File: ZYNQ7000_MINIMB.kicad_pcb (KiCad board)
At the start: 4 copper layers, 86 x 68.9 mm, 125 parts, among them J1 Conn_02x50_Odd_Even, J10 Conn_02x20_Odd_Even, J11 USB_A_Stacked, J12 Conn_01x40, J2 Conn_02x50_Odd_Even, J3 ZYNQ_JTAG, J5 USB_C_Receptacle_USB2.0, J6 HDMI_A, J8 USB_A_Stacked, J9 USB_C_Receptacle_USB2.0, SW2 SW_DIP_x01, SW5 SW_DIP_x02, U1 HR911130A, U2 CP2102N-A01-GQFN28, U4 TXS02612RTWR, U5 TF_Card, U6 TXS0108EPWR, U7 USB3320, U8 TPS2051BDBV, U9 GL850G, Y1 24Mhz, Y2 12Mhz

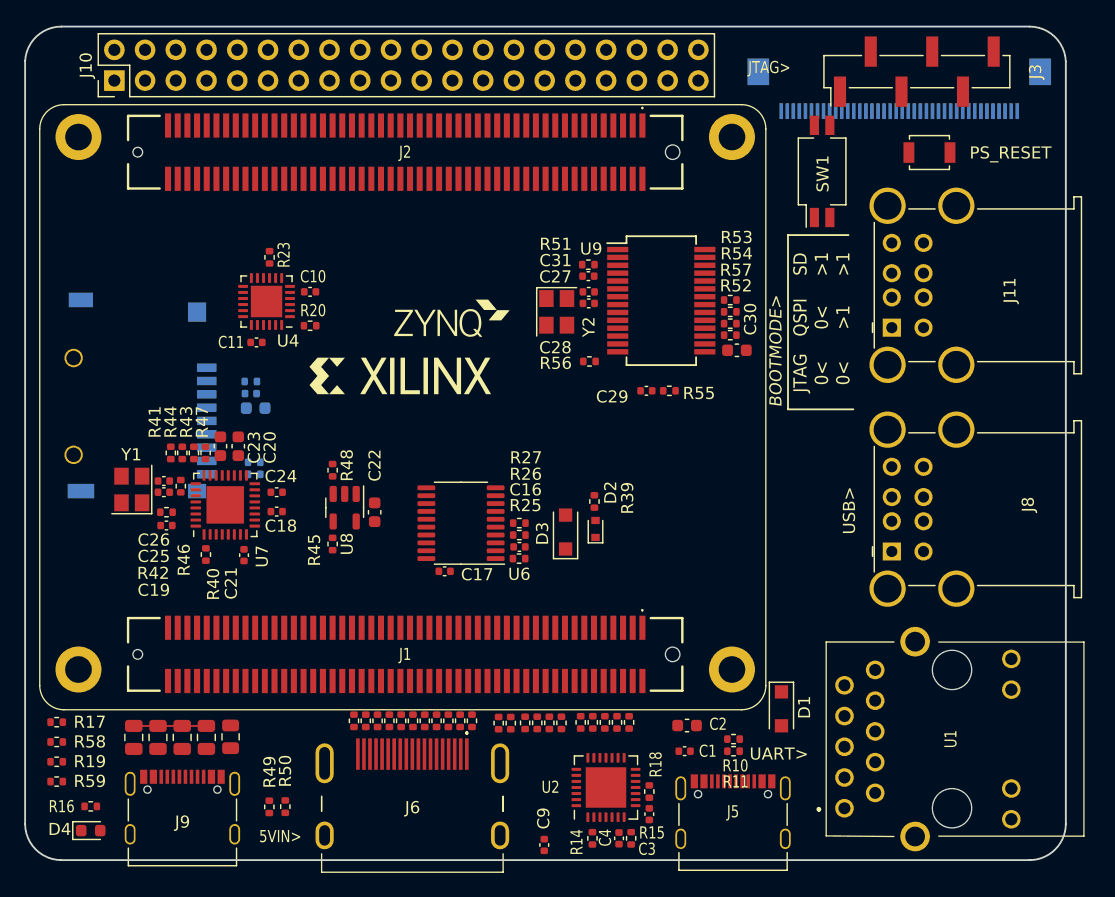
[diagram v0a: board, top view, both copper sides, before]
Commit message: update layout
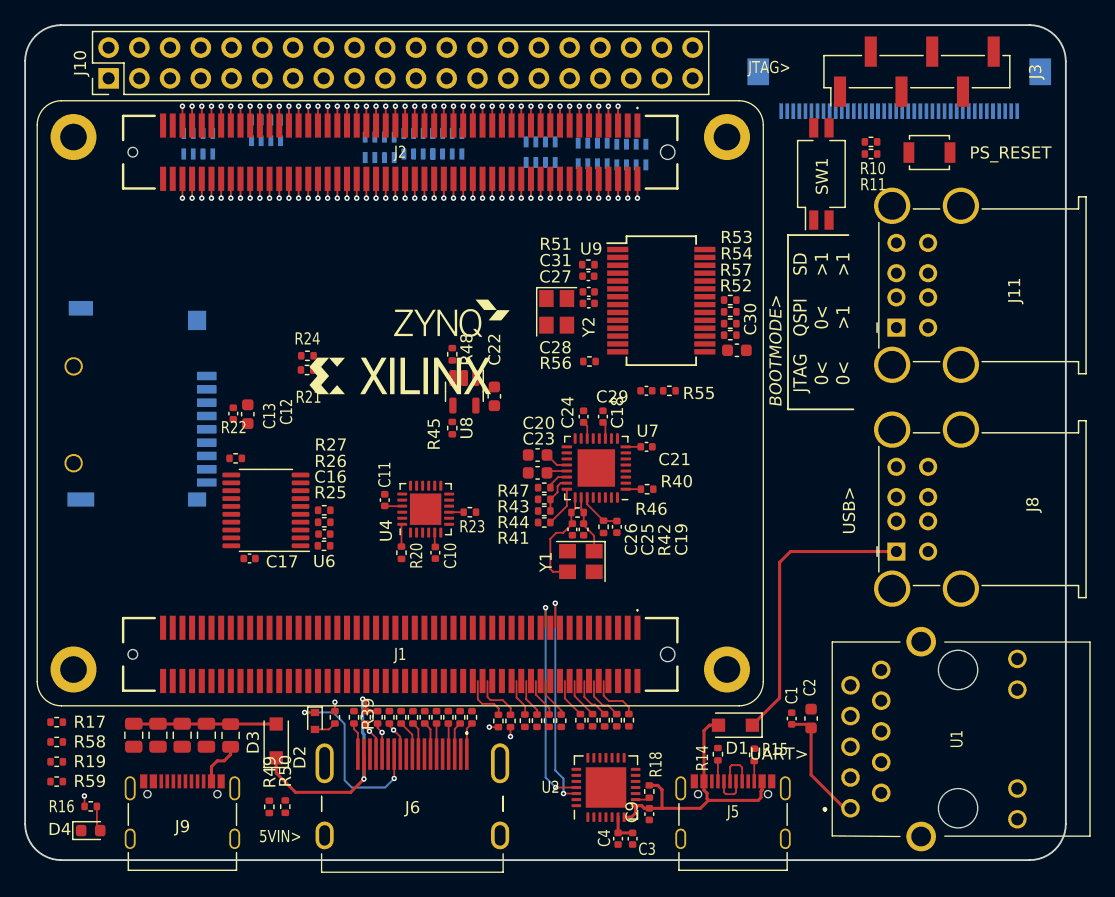
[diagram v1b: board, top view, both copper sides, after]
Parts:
- added RN1: R_Pack04, Resistor_SMD:R_Array_Concave_4x0603, B.Cu at (120.1, 61.7)
- added RN2: R_Pack04, Resistor_SMD:R_Array_Concave_4x0603, B.Cu at (116.9, 61.6)
- added RN3: R_Pack04, Resistor_SMD:R_Array_Concave_4x0603, B.Cu at (104.9, 60.8)
- added RN4: R_Pack04, Resistor_SMD:R_Array_Concave_4x0603, B.Cu at (112.6, 61.5)
- added RN5: R_Pack04, Resistor_SMD:R_Array_Concave_4x0603, B.Cu at (102.5, 60.8)
- added RN6: R_Pack04, Resistor_SMD:R_Array_Concave_4x0603, B.Cu at (99.3, 61.1)
- added RN7: R_Pack04, Resistor_SMD:R_Array_Concave_4x0603, B.Cu at (84.3, 60.8)
- added RN8: R_Pack04, Resistor_SMD:R_Array_Concave_4x0603, B.Cu at (89.9, 59.7)
- C12, C13, R21, R22, R24: moved to F.Cu
- moved R10 50.6 mm to (139.9, 60.6)
- moved R11 50.6 mm to (139.9, 61.6)
- moved Y1 37.6 mm to (115.9, 95.3), turned to 180 degrees
- moved C19 37.2 mm to (118.9, 92.5), turned to -90 degrees
- moved R40 36.9 mm to (121.4, 89.3), turned to 180 degrees
- moved R42 36.1 mm to (117.8, 92.5), turned to -90 degrees
- moved C25 34.8 mm to (116.2, 92.7), turned to -90 degrees
- moved C21 34.4 mm to (121.3, 85.8), turned to 0 degrees
- moved C26 34.0 mm to (115.2, 92.7), turned to -90 degrees
- moved R46 32.9 mm to (115.7, 91.3), turned to 0 degrees
- moved R41 31.4 mm to (112.9, 92.1), turned to 0 degrees
- moved U7 30.8 mm to (117.2, 87.6), turned to 180 degrees
- moved R44 30.3 mm to (112.9, 91.2), turned to 180 degrees
- moved D3 29.5 mm to (90.8, 110.2)
- moved R43 29.2 mm to (112.9, 90.2), turned to 180 degrees
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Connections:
- C3 pad 2: GND2 -> GND
- C4 pad 2: GND2 -> GND
- C9 pad 2: GND2 -> GND
- J10 pad 10: /B35_L7N -> Net-(J10-Pad10)
- J10 pad 13: /B34_L7P -> Net-(J10-Pad13)
- J10 pad 14: /B34_L7N -> Net-(J10-Pad14)
- J10 pad 15: /B34_L10P -> Net-(J10-Pad15)
- J10 pad 16: /B34_L10N -> Net-(J10-Pad16)
- J10 pad 17: /B34_L8P -> Net-(J10-Pad17)
- J10 pad 18: /B34_L8N -> Net-(J10-Pad18)
- J10 pad 19: /B34_L9P -> Net-(J10-Pad19)
- J10 pad 20: /B34_L9N -> Net-(J10-Pad20)
- J10 pad 21: /B34_L2P -> Net-(J10-Pad21)
- J10 pad 22: /B34_L2N -> Net-(J10-Pad22)
- J10 pad 23: /B34_L1P -> Net-(J10-Pad23)
- J10 pad 24: /B34_L1N -> Net-(J10-Pad24)
- J10 pad 27: /B13_L11P -> Net-(J10-Pad27)
- J10 pad 28: /B13_L11N -> Net-(J10-Pad28)
- J10 pad 29: /B13_L19P -> Net-(J10-Pad29)
- J10 pad 3: /B35_L11P -> Net-(J10-Pad3)
- J10 pad 30: /B13_L19N -> Net-(J10-Pad30)
- J10 pad 31: /B13_L18P -> Net-(J10-Pad31)
- J10 pad 32: /B13_L18N -> Net-(J10-Pad32)
- J10 pad 33: /B13_L16P -> Net-(J10-Pad33)
- J10 pad 34: /B13_L16N -> Net-(J10-Pad34)
- J10 pad 35: /B13_L14P -> Net-(J10-Pad35)
- J10 pad 36: /B13_L14N -> Net-(J10-Pad36)
- J10 pad 37: /B13_L13P -> Net-(J10-Pad37)
- J10 pad 38: /B13_L13N -> Net-(J10-Pad38)
- J10 pad 4: /B35_L11N -> Net-(J10-Pad4)
- J10 pad 5: /B35_L21P -> Net-(J10-Pad5)
- J10 pad 6: /B35_L21N -> Net-(J10-Pad6)
- J10 pad 7: /B35_L9P -> Net-(J10-Pad7)
- J10 pad 8: /B35_L9N -> Net-(J10-Pad8)
- J10 pad 9: /B35_L7P -> Net-(J10-Pad9)
- J5 pad A1: GND2 -> GND
- J5 pad A12: GND2 -> GND
- J5 pad B1: GND2 -> GND
- J5 pad B12: GND2 -> GND
- J5 pad S1: GND2 -> GND
- R14 pad 1: GND2 -> GND
- R15 pad 1: GND2 -> GND
- U2 pad 29: GND2 -> GND
- U2 pad 3: GND2 -> GND
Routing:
- net /USB_5V: track 0.00 -> 24.0 mm
- net Net-(C3-Pad1): track 0.00 -> 23.9 mm
- net /hdmi/HDMI5VD: track 0.00 -> 20.4 mm, vias 0 -> 2
- net /B0MIO14: track 0.00 -> 19.1 mm, vias 0 -> 2
- net /B0MIO15: track 0.00 -> 18.6 mm, vias 0 -> 2
- net /B35_L3P: track 0.00 -> 15.9 mm, vias 0 -> 2
- net Net-(C1-Pad1): track 0.00 -> 9.50 mm
- net Net-(C26-Pad1): track 0.00 -> 8.68 mm
- net GND: track 0.00 -> 8.00 mm, vias 0 -> 5
- net /VDD5VD: track 6.00 -> 12.6 mm, vias 0 -> 1
- net /VDD1V8D: track 0.00 -> 5.31 mm
- net Net-(C25-Pad1): track 0.00 -> 4.89 mm
- net /PHY_LED0: track 0.00 -> 4.36 mm
- net /B0MIO06: track 0.00 -> 4.26 mm
- net /PHY_LED1: track 0.00 -> 4.25 mm
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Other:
- board size 86 x 68.9 mm -> 86 x 69 mm

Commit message: update sch&layout
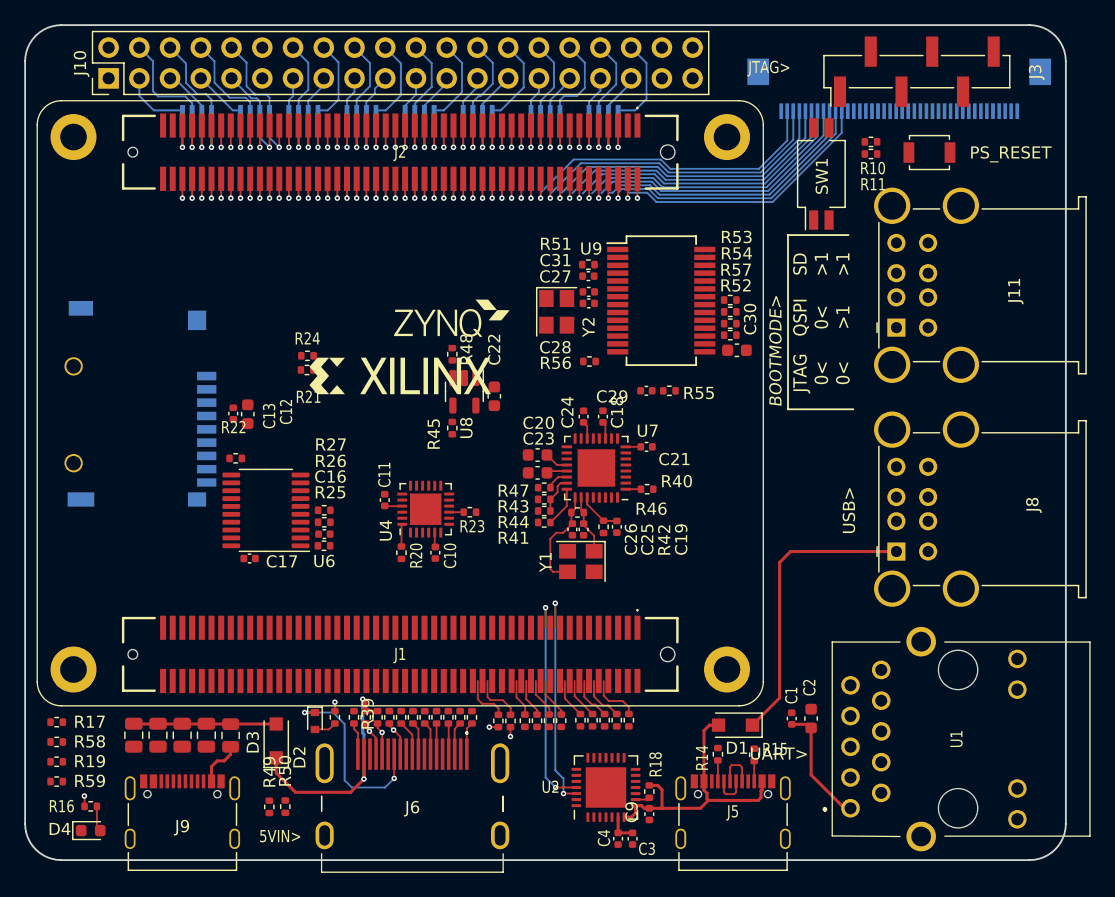
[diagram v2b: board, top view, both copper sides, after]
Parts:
- moved RN6 6.67 mm to (93.0, 58.9), turned to -90 degrees
- moved RN4 5.81 mm to (107.4, 58.9), turned to -90 degrees
- moved RN5 5.07 mm to (97.8, 58.9), turned to -90 degrees
- moved RN2 4.74 mm to (113.0, 58.9), turned to -90 degrees
- moved RN1 3.62 mm to (117.8, 58.9), turned to -90 degrees
- moved RN3 2.98 mm to (102.6, 58.9), turned to -90 degrees
- moved RN7 1.90 mm to (84.2, 58.9)
- moved RN8 1.20 mm to (89.0, 58.9)
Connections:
- net Net-(J10-Pad23) renamed /P23
- net Net-(J10-Pad5) renamed /P5
- J10 pad 10: Net-(J10-Pad10) -> /P10
- J10 pad 13: Net-(J10-Pad13) -> /P13
- J10 pad 14: Net-(J10-Pad14) -> /P14
- J10 pad 15: Net-(J10-Pad15) -> /P15
- J10 pad 16: Net-(J10-Pad16) -> /P16
- J10 pad 17: Net-(J10-Pad17) -> /P17
- J10 pad 18: Net-(J10-Pad18) -> /P18
- J10 pad 19: Net-(J10-Pad19) -> /P19
- J10 pad 20: Net-(J10-Pad20) -> /P20
- J10 pad 21: Net-(J10-Pad21) -> /P21
- J10 pad 22: Net-(J10-Pad22) -> /P22
- J10 pad 24: Net-(J10-Pad24) -> /P24
- J10 pad 25: GND -> /P25
- J10 pad 26: GND -> /P26
- J10 pad 27: Net-(J10-Pad27) -> /P27
- J10 pad 28: Net-(J10-Pad28) -> /P28
- J10 pad 29: Net-(J10-Pad29) -> /P29
- J10 pad 3: Net-(J10-Pad3) -> /P3
- J10 pad 30: Net-(J10-Pad30) -> /P30
- J10 pad 31: Net-(J10-Pad31) -> /P31
- J10 pad 32: Net-(J10-Pad32) -> /P32
- J10 pad 33: Net-(J10-Pad33) -> /P33
- J10 pad 34: Net-(J10-Pad34) -> /P34
- J10 pad 35: Net-(J10-Pad35) -> /P35
- J10 pad 36: Net-(J10-Pad36) -> /P36
- J10 pad 37: Net-(J10-Pad37) -> unconnected-(J10-Pad37)
- J10 pad 38: Net-(J10-Pad38) -> unconnected-(J10-Pad38)
- J10 pad 4: Net-(J10-Pad4) -> /P4
- J10 pad 6: Net-(J10-Pad6) -> /P6
- J10 pad 7: Net-(J10-Pad7) -> /P7
- J10 pad 8: Net-(J10-Pad8) -> /P8
- J10 pad 9: Net-(J10-Pad9) -> /P9
- J12 pad 1: unconnected-(J12-Pad1) -> /VDD5VD
- J12 pad 10: unconnected-(J12-Pad10) -> /B34_L14P
- J12 pad 11: unconnected-(J12-Pad11) -> /B34_L14N
- J12 pad 12: unconnected-(J12-Pad12) -> /B34_L13P
- J12 pad 13: unconnected-(J12-Pad13) -> /B34_L13N
- J12 pad 14: unconnected-(J12-Pad14) -> /B34_L23P
- J12 pad 15: unconnected-(J12-Pad15) -> /B34_L23N
- J12 pad 16: unconnected-(J12-Pad16) -> /B34_L6P
- J12 pad 17: unconnected-(J12-Pad17) -> /B34_L6N
- J12 pad 18: unconnected-(J12-Pad18) -> /B34_L20P
- J12 pad 19: unconnected-(J12-Pad19) -> /B34_L20N
- J12 pad 2: unconnected-(J12-Pad2) -> /B35_L17P
- J12 pad 20: unconnected-(J12-Pad20) -> /B34_L22P
- J12 pad 21: unconnected-(J12-Pad21) -> /B34_L22N
- J12 pad 22: unconnected-(J12-Pad22) -> /B34_L18P
- J12 pad 23: unconnected-(J12-Pad23) -> /B34_L18N
- J12 pad 24: unconnected-(J12-Pad24) -> /B34_L21P
- J12 pad 25: unconnected-(J12-Pad25) -> /B34_L21N
- J12 pad 26: unconnected-(J12-Pad26) -> /B34_L11P
- J12 pad 27: unconnected-(J12-Pad27) -> /B34_L11N
- J12 pad 28: unconnected-(J12-Pad28) -> /B34_L5P
- J12 pad 29: unconnected-(J12-Pad29) -> /B34_L5N
- J12 pad 3: unconnected-(J12-Pad3) -> /B35_L17N
- J12 pad 30: unconnected-(J12-Pad30) -> /B34_L3P
- J12 pad 31: unconnected-(J12-Pad31) -> /B34_L3N
- J12 pad 32: unconnected-(J12-Pad32) -> /B34_L4P
- J12 pad 33: unconnected-(J12-Pad33) -> /B34_L4N
- J12 pad 34: unconnected-(J12-Pad34) -> /B13_L12P
- J12 pad 35: unconnected-(J12-Pad35) -> /B13_L12N
- J12 pad 36: unconnected-(J12-Pad36) -> /B13_L20P
- J12 pad 37: unconnected-(J12-Pad37) -> /B13_L20N
- J12 pad 38: unconnected-(J12-Pad38) -> /B13_L21P
- J12 pad 39: unconnected-(J12-Pad39) -> /B13_L21N
- J12 pad 4: unconnected-(J12-Pad4) -> /B35_L23P
- J12 pad 40: unconnected-(J12-Pad40) -> GND
- J12 pad 5: unconnected-(J12-Pad5) -> /B35_L23N
- J12 pad 6: unconnected-(J12-Pad6) -> /B35_L12P
- J12 pad 7: unconnected-(J12-Pad7) -> /B35_L12N
- J12 pad 8: unconnected-(J12-Pad8) -> /B35_L8P
- J12 pad 9: unconnected-(J12-Pad9) -> /B35_L8N
- RN1 pad 1: Net-(J10-Pad37) -> /P33
- RN1 pad 2: Net-(J10-Pad35) -> /P34
- RN1 pad 3: Net-(J10-Pad33) -> /P35
- RN1 pad 4: Net-(J10-Pad31) -> /P36
- RN1 pad 5: /B13_L18P -> /B13_L13N
- RN1 pad 6: /B13_L16P -> /B13_L13P
- RN1 pad 7: /B13_L14P -> /B13_L14N
- RN1 pad 8: /B13_L13P -> /B13_L14P
- RN2 pad 1: /B13_L13N -> /P29
- RN2 pad 2: /B13_L14N -> /P30
- RN2 pad 3: /B13_L16N -> /P31
- RN2 pad 4: /B13_L18N -> /P32
- RN2 pad 5: Net-(J10-Pad32) -> /B13_L18N
- RN2 pad 6: Net-(J10-Pad34) -> /B13_L18P
- RN2 pad 7: Net-(J10-Pad36) -> /B13_L19N
- RN2 pad 8: Net-(J10-Pad38) -> /B13_L19P
- RN3 pad 1: Net-(J10-Pad29) -> /P21
- RN3 pad 2: Net-(J10-Pad27) -> /P22
- RN3 pad 4: Net-(J10-Pad21) -> /P24
- RN3 pad 5: /B34_L2P -> /B34_L8N
- RN3 pad 6: /B34_L1P -> /B34_L8P
- RN3 pad 7: /B13_L11P -> /B34_L10N
- RN3 pad 8: /B13_L19P -> /B34_L10P
- RN4 pad 1: /B13_L19N -> /P25
- RN4 pad 2: /B13_L11N -> /P26
- RN4 pad 3: /B34_L1N -> /P27
- RN4 pad 4: /B34_L2N -> /P28
- RN4 pad 5: Net-(J10-Pad22) -> /B34_L1N
- RN4 pad 6: Net-(J10-Pad24) -> /B34_L1P
- RN4 pad 7: Net-(J10-Pad28) -> /B34_L2N
- RN4 pad 8: Net-(J10-Pad30) -> /B34_L2P
- RN5 pad 1: Net-(J10-Pad19) -> /P17
- RN5 pad 2: Net-(J10-Pad17) -> /P18
- RN5 pad 3: Net-(J10-Pad15) -> /P19
- RN5 pad 4: Net-(J10-Pad13) -> /P20
- RN5 pad 5: /B34_L7P -> /B34_L17N
- RN5 pad 6: /B34_L10P -> /B34_L17P
- RN5 pad 7: /B34_L8P -> /B34_L16N
- RN5 pad 8: /B34_L9P -> /B34_L16P
- RN6 pad 1: /B34_L9N -> /P13
- RN6 pad 2: /B34_L8N -> /P14
- RN6 pad 3: /B34_L10N -> /P15
- RN6 pad 4: /B34_L7N -> /P16
- RN6 pad 5: Net-(J10-Pad14) -> /B34_L24N
- RN6 pad 6: Net-(J10-Pad16) -> /B34_L24P
- RN6 pad 7: Net-(J10-Pad18) -> /B34_L15N
- RN6 pad 8: Net-(J10-Pad20) -> /B34_L15P
- RN7 pad 1: Net-(J10-Pad9) -> /P3
- RN7 pad 2: Net-(J10-Pad7) -> /P4
- RN7 pad 4: Net-(J10-Pad3) -> /P6
- RN7 pad 5: /B35_L11P -> /B35_L21N
- RN7 pad 7: /B35_L9P -> /B35_L11N
- RN7 pad 8: /B35_L7P -> /B35_L11P
- RN8 pad 1: /B35_L7N -> /P7
- RN8 pad 2: /B35_L9N -> /P8
- RN8 pad 3: /B35_L21N -> /P9
- RN8 pad 4: /B35_L11N -> /P10
- RN8 pad 5: Net-(J10-Pad4) -> /B34_IO25
- RN8 pad 6: Net-(J10-Pad6) -> /B34_L12N
- RN8 pad 7: Net-(J10-Pad8) -> /B35_L7N
- RN8 pad 8: Net-(J10-Pad10) -> /B35_L7P
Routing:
- net /B35_L17P: track 1.60 -> 26.8 mm
- net /B35_L17N: track 1.60 -> 26.4 mm
- net /B35_L23P: track 1.60 -> 26.0 mm
- net /B35_L23N: track 1.60 -> 25.6 mm
- net /B35_L12P: track 1.60 -> 25.2 mm
- net /B35_L12N: track 1.60 -> 24.9 mm
- net /B35_L8P: track 1.60 -> 24.6 mm
- net /B35_L8N: track 1.60 -> 24.4 mm
- net /B34_L14P: track 1.60 -> 24.1 mm
- net /B34_L14N: track 1.60 -> 23.8 mm
- net /P4: track 0.00 -> 8.31 mm
- net /P8: track 0.00 -> 7.67 mm
- net /P36: track 0.00 -> 7.51 mm
- net /P28: track 0.00 -> 7.21 mm
- net /P32: track 0.00 -> 7.17 mm
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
